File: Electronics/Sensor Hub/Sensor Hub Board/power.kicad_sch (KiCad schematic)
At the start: 25 parts, among them IC201 TPS54295PWPR, J2 Screw_Terminal_01x02, J202 Conn_01x02_Pin, J203 Conn_01x02_Pin, J204 Conn_01x02_Pin

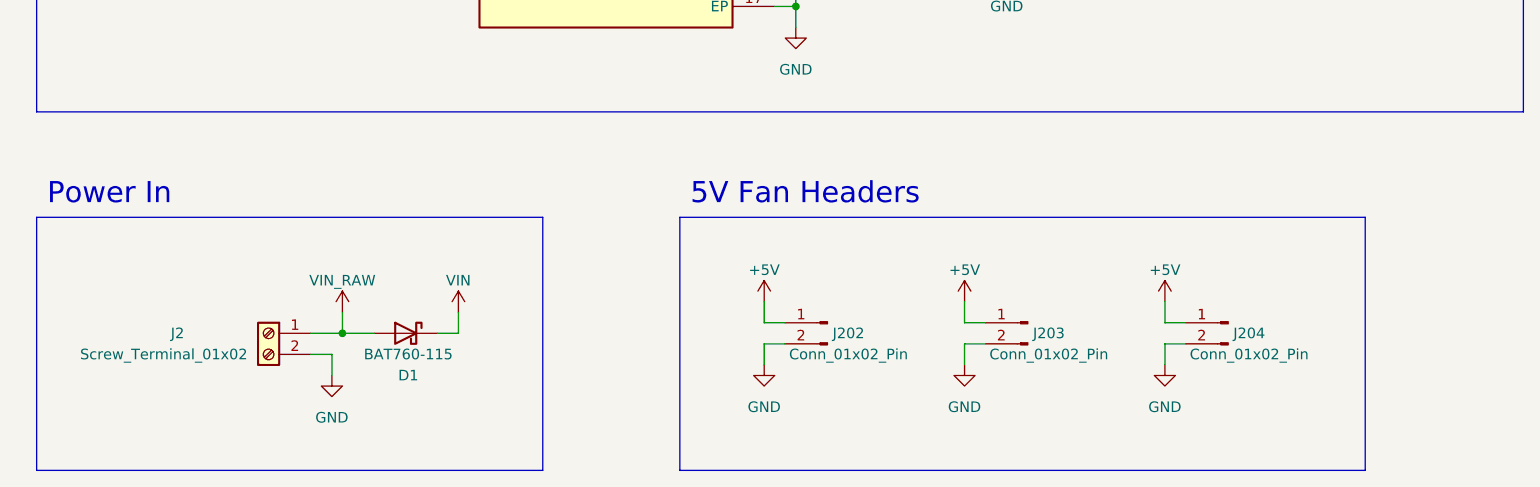
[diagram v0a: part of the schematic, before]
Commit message: PCB Schematics finished
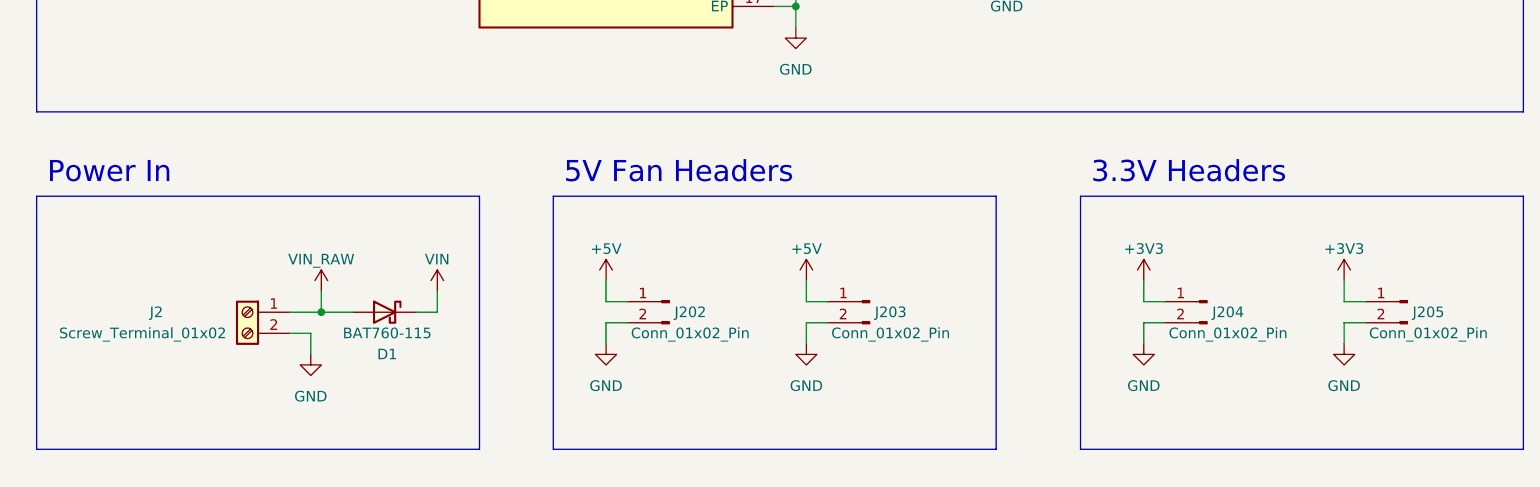
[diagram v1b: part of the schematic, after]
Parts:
- added J205: Conn_01x02_Pin, Connector_PinHeader_2.54mm:PinHeader_1x02_P2.54mm_Vertical, symbol Connector:Conn_01x02_Pin
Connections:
- net +3V3: now also J204.1 (Pin_1), J205.1 (Pin_1)
- net +5V: no longer J204.1 (Pin_1)
- net GND: now also J205.2 (Pin_2)
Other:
- note added: "3.3V Headers"
- moved on the sheet: D1, J2, J202, J203, J204
